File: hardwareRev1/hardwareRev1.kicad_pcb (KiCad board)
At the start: 2 copper layers, 0 parts

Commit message: board is almost done. Commiting before I destroy all my work...
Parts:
- added A1: GPSAnt, hardwareRev1:GPSAnt, F.Cu at (143.0, 84.0)
- added C1: C, Capacitors_SMD:C_0603, B.Cu at (167.7, 46.0)
- added C10: C, Capacitors_SMD:C_0603, F.Cu at (190.8, 41.8)
- added C11: C, Capacitors_SMD:C_0603, F.Cu at (178.8, 55.6)
- added C12: C, Capacitors_SMD:C_0603, B.Cu at (165.2, 56.8)
- added C13: C, Capacitors_SMD:C_0603, F.Cu at (175.1, 66.8)
- added C2: C, Capacitors_SMD:C_0603, F.Cu at (161.8, 62.6)
- added C3: C, Capacitors_SMD:C_0603, F.Cu at (175.1, 75.4)
- added C4: C, Capacitors_SMD:C_0603, F.Cu at (171.7, 72.6)
- added C5: C, Capacitors_SMD:C_0603, F.Cu at (180.0, 65.8)
- added C6: C, Capacitors_SMD:C_0603, F.Cu at (221.0, 53.0)
- added C7: CAPAPOL, Capacitors_SMD:C_0603, F.Cu at (221.0, 49.0)
- added C8: C, Capacitors_SMD:C_0603, B.Cu at (168.0, 76.0)
- added C9: C, Capacitors_SMD:C_0603, B.Cu at (171.0, 76.0)
- added D1: LED, LEDs:LED-0805, F.Cu at (167.6, 45.7)
- added D2: LED, LEDs:LED-0805, F.Cu at (169.3, 45.7)
- added D3: LED, LEDs:LED-0805, F.Cu at (171.1, 45.7)
- added D4: LED, LEDs:LED-0805, F.Cu at (172.8, 45.8)
- added D5: DIODE, Diodes_ThroughHole:Diode_DO-41_SOD81_Vertical_AnodeUp, F.Cu at (175.0, 46.0)
- added J1: MicroSD, Footprints:MICRO_SD_HINGE_AMP, B.Cu at (183.0, 72.0)
- added J2: SMA, hardwareRev1:SMA, F.Cu at (213.0, 74.0)
- added JMP1: SJMPOpen, SparkFun:SparkFun-SJ_2S-NO, B.Cu at (167.8, 48.6)
- added JMP2: SJMPOpen, SparkFun:SparkFun-SJ_2S-NO, F.Cu at (165.0, 45.0)
- added JMP3: SJMPOpen, SparkFun:SparkFun-SJ_2S-NO, F.Cu at (165.0, 47.0)
- added K1: PWMOut, Footprints:CONN_1x3, F.Cu at (146.8, 45.6)
- added K2: ADC1, Footprints:CONN_1x3, F.Cu at (146.8, 42.0)
- added P1: UART, Footprints:CONN_1x4, F.Cu at (148.0, 49.0)
- added P10: ID, Measurement_Points:Measurement_Point_Round-SMD-Pad_Small, B.Cu at (157.7, 47.2)
- added P2: I2C, Footprints:CONN_1x4, F.Cu at (148.0, 52.0)
- added P3: ADC2, Footprints:CONN_1x5, F.Cu at (143.8, 60.4)
- added P4: CONN_7, Footprints:CONN_1x7, F.Cu at (147.1, 63.0)
- added P5: CONN_5X2, hardwareRev1:CortexDebug, F.Cu at (192.2, 70.8)
- added P6: CONN_11X2, hardwareRev1:1.27mmPitchHeader11X2, F.Cu at (172.0, 42.0)
- added P7: GPSDM, Measurement_Points:Measurement_Point_Round-SMD-Pad_Small, F.Cu at (164.0, 67.0)
- added P8: GPSDP, Measurement_Points:Measurement_Point_Round-SMD-Pad_Small, F.Cu at (162.0, 67.0)
- added P9: USBPW, Measurement_Points:Measurement_Point_Round-SMD-Pad_Small, F.Cu at (161.7, 47.4)
- added Q1: MOS_P_NUM, SMD_Packages:SOT-323, B.Cu at (170.0, 72.0)
- added R1: R, Resistors_SMD:R_0603, F.Cu at (163.4, 62.6)
- added R10: R, Resistors_SMD:R_0603, F.Cu at (194.2, 41.5)
- added R11: R, Resistors_SMD:R_0603, F.Cu at (190.8, 39.8)
- added R12: R, Resistors_SMD:R_0603, F.Cu at (193.7, 74.8)
- added R13: R, Resistors_SMD:R_0603, B.Cu at (167.7, 73.0)
- added R2: R, Resistors_SMD:R_0603, F.Cu at (178.0, 49.0)
- added R3: R, Resistors_SMD:R_0603, F.Cu at (167.6, 49.2)
- added R4: R, Resistors_SMD:R_0603, F.Cu at (169.5, 49.2)
- added R5: R, Resistors_SMD:R_0603, F.Cu at (171.1, 49.2)
- added R6: R, Resistors_SMD:R_0603, F.Cu at (173.1, 49.2)
- added R7: R, Resistors_SMD:R_0603, F.Cu at (178.7, 70.8)
- added R8: R, Resistors_SMD:R_0603, F.Cu at (180.0, 68.0)
- added R9: R, Resistors_SMD:R_0603, F.Cu at (183.5, 65.8)
- added RF1: NEO7, hardwareRev1:NEO-7, F.Cu at (153.0, 83.0)
- added RF2: DRA818, dra818:DRA818, F.Cu at (182.0, 63.0)
- added S1: TAC_SWITCHSMD, SparkFun:SparkFun-TACTILE_SWITCH_SMD, B.Cu at (187.0, 61.0)
- added S2: TAC_SWITCHSMD, SparkFun:SparkFun-TACTILE_SWITCH_SMD, F.Cu at (156.4, 58.0)
- added U1: MKL26Z128VLH4, w_smd_lqfp:lqfp64, F.Cu at (171.0, 59.0)
- added U2: 24C16, Housings_SOIC:SOIC-8_3.9x4.9mm_Pitch1.27mm, B.Cu at (155.1, 59.0)
- added U3: MICRO-B_USB, USB:USB micro B female, F.Cu at (159.0, 42.0)
- added X1: CRYSTAL_ABM3C, open-project:CRYSTAL_ABM3C, F.Cu at (175.2, 70.8)
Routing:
- net GND: track 0.00 -> 333.9 mm, vias 0 -> 68
- net +3.3V: track 0.00 -> 171.9 mm, vias 0 -> 3
- net /internalSPI0MOSI: track 0.00 -> 47.7 mm, vias 0 -> 3
- net /DRAPttIRQ: track 0.00 -> 43.8 mm, vias 0 -> 2
- net /internalI2C0SCL: track 0.00 -> 42.5 mm, vias 0 -> 3
- net /DRAHLCSel: track 0.00 -> 42.2 mm, vias 0 -> 2
- net /DRATx: track 0.00 -> 39.5 mm, vias 0 -> 4
- net /DRAPD: track 0.00 -> 38.5 mm, vias 0 -> 2
- net /externalSPI1SCK: track 0.00 -> 36.9 mm, vias 0 -> 1
- net /GPSTX: track 0.00 -> 34.6 mm, vias 0 -> 2
- net /DRARx: track 0.00 -> 34.6 mm, vias 0 -> 2
- net /externalSPI1CS1: track 0.00 -> 34.5 mm, vias 0 -> 2
- net /externalPWMOut: track 0.00 -> 34.4 mm, vias 0 -> 2
- net /GPSRX: track 0.00 -> 34.2 mm, vias 0 -> 2
- net /externalSPI1PCS0: track 0.00 -> 32.4 mm, vias 0 -> 2
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- added copper zone on B.Cu, net GND
- added copper zone on F.Cu, net GND
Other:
- net class Default: clearance 0.2 -> 0.1524; trace_width 0.25 -> 0.1524
- rule pad_to_mask_clearance: 0 -> 0.2
- rule trace_clearance: 0.2 -> 0.1524
- rule trace_min: 0.2 -> 0.1524

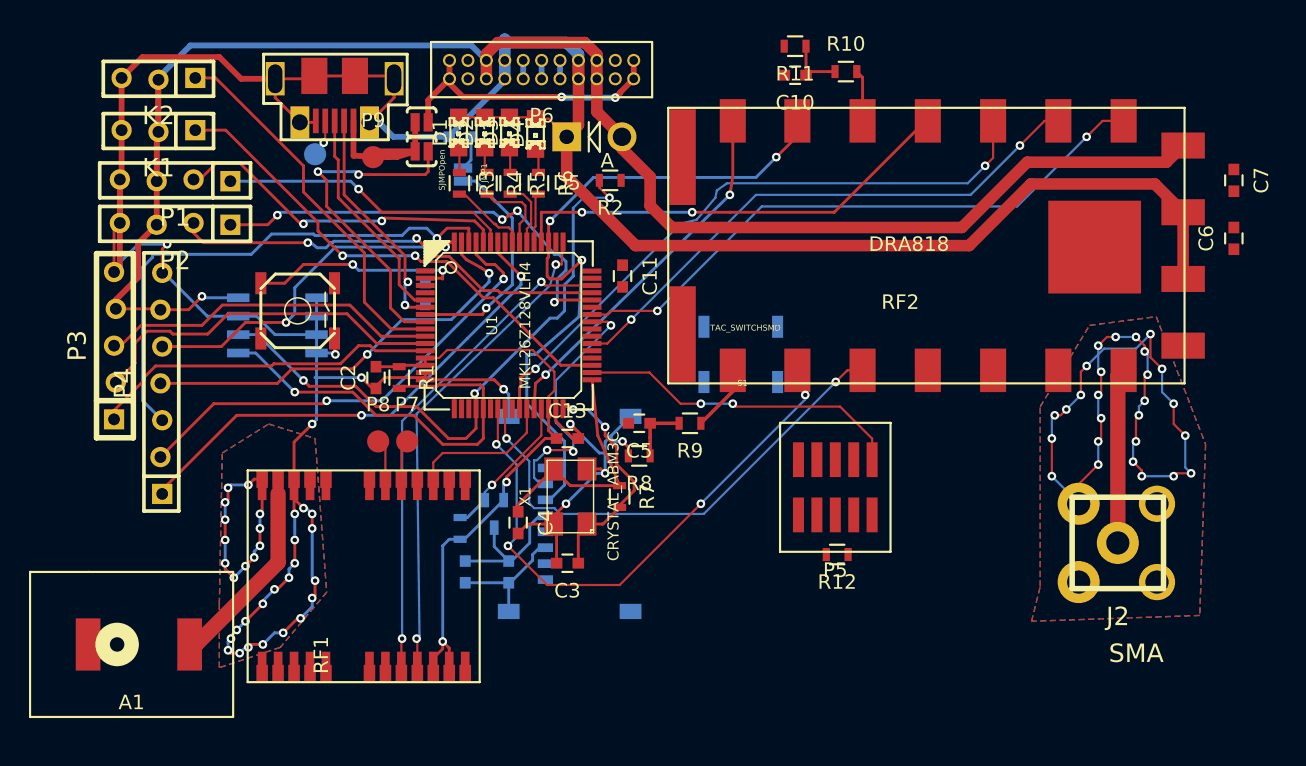
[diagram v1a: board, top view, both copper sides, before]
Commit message: went further.
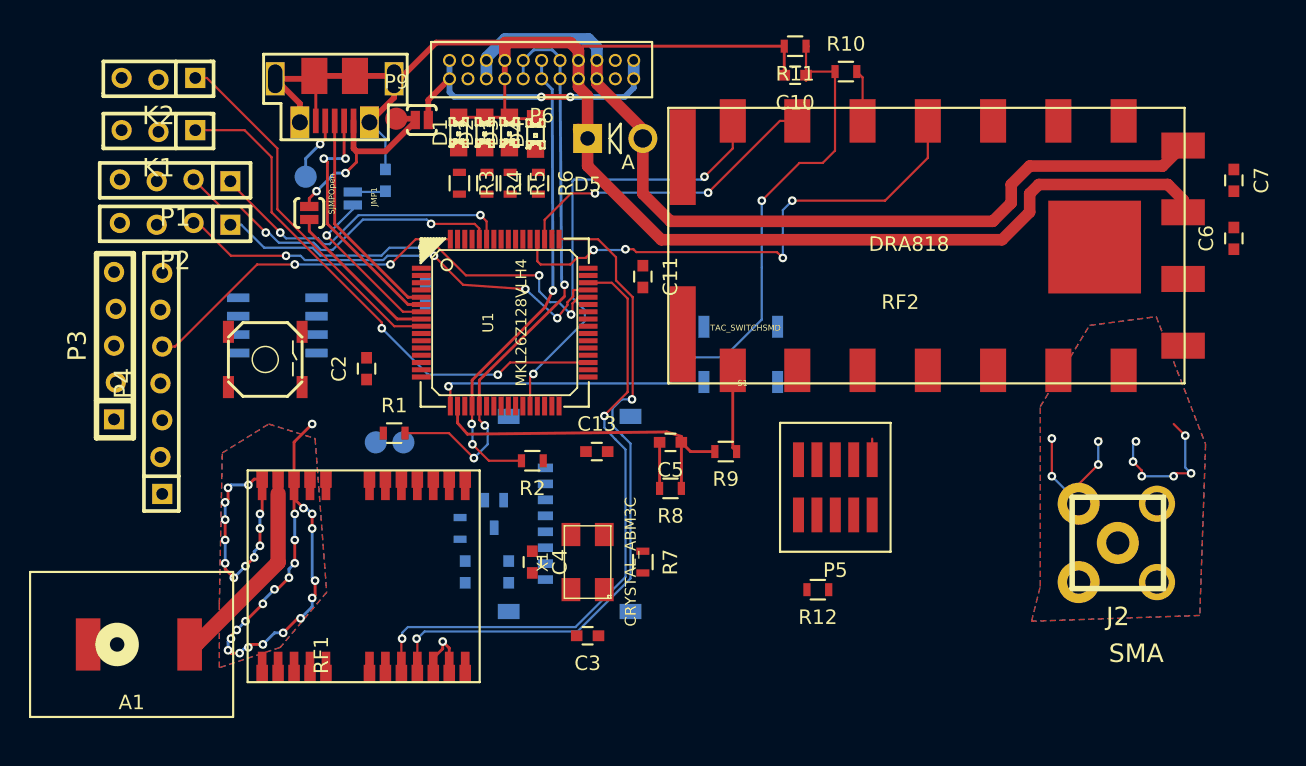
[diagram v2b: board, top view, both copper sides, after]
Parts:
- P7, P8: moved to B.Cu
- moved R2 20.1 mm to (172.6, 68.3)
- moved JMP3 8.84 mm to (157.2, 51.2), turned to 270 degrees
- moved JMP1 7.78 mm to (160.2, 50.2)
- moved C1 5.96 mm to (162.5, 49.0), turned to 270 degrees
- moved C3 5.19 mm to (176.4, 80.4)
- moved R7 4.79 mm to (180.2, 75.3)
- moved X1 4.67 mm to (176.4, 75.3)
- moved S2 4.03 mm to (154.2, 61.4)
- moved R1 3.85 mm to (163.1, 66.4), turned to 0 degrees
- moved R9 3.14 mm to (186.0, 67.7)
- moved R8 3.11 mm to (182.2, 70.2)
- moved P9 3.10 mm to (163.2, 44.8)
- moved C4 2.89 mm to (172.6, 75.3)
- moved R12 2.77 mm to (192.3, 77.2)
- moved C5 2.52 mm to (182.2, 67.1)
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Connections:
- P6 pad 10: /PWRSDA -> /internalI2C0SDA
- P6 pad 11: /PwrCLK -> /internalI2C0SCL
- P6 pad 12: /PwrCLK -> /internalI2C0SCL
- P6 pad 13: /PWRSDA -> /internalI2C0SDA
- P6 pad 14: /PWRSDA -> /internalI2C0SDA
- P6 pad 9: /PWRSDA -> /internalI2C0SDA
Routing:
- net GND: track 333.9 -> 183.8 mm, vias 68 -> 37
- net +3.3V: track 171.9 -> 65.0 mm, vias 3 -> 1
- net /DRAAFOut: track 4.75 -> 49.8 mm, vias 0 -> 2
- net /DRAPttIRQ: track 43.8 -> 0.00 mm, vias 2 -> 0
- net /DRAHLCSel: track 42.2 -> 0.00 mm, vias 2 -> 0
- net /DRATx: track 39.5 -> 0.00 mm, vias 4 -> 0
- net /DRAPD: track 38.5 -> 0.00 mm, vias 2 -> 0
- net /externalSPI1SCK: track 36.9 -> 0.00 mm, vias 1 -> 0
- net /DRARx: track 34.6 -> 0.00 mm, vias 2 -> 0
- net /externalSPI1CS1: track 34.5 -> 0.28 mm, vias 2 -> 0
- net /externalSPI1PCS0: track 32.4 -> 0.00 mm, vias 2 -> 0
- net /externalSPI1MOSI: track 29.3 -> 0.00 mm, vias 2 -> 0
- net /internalSPI0MOSI: track 47.7 -> 21.6 mm, vias 3 -> 2
- net /externalADC3: track 25.1 -> 0.00 mm
- net /externalADC4: track 24.2 -> 0.00 mm
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
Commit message: better routed it.
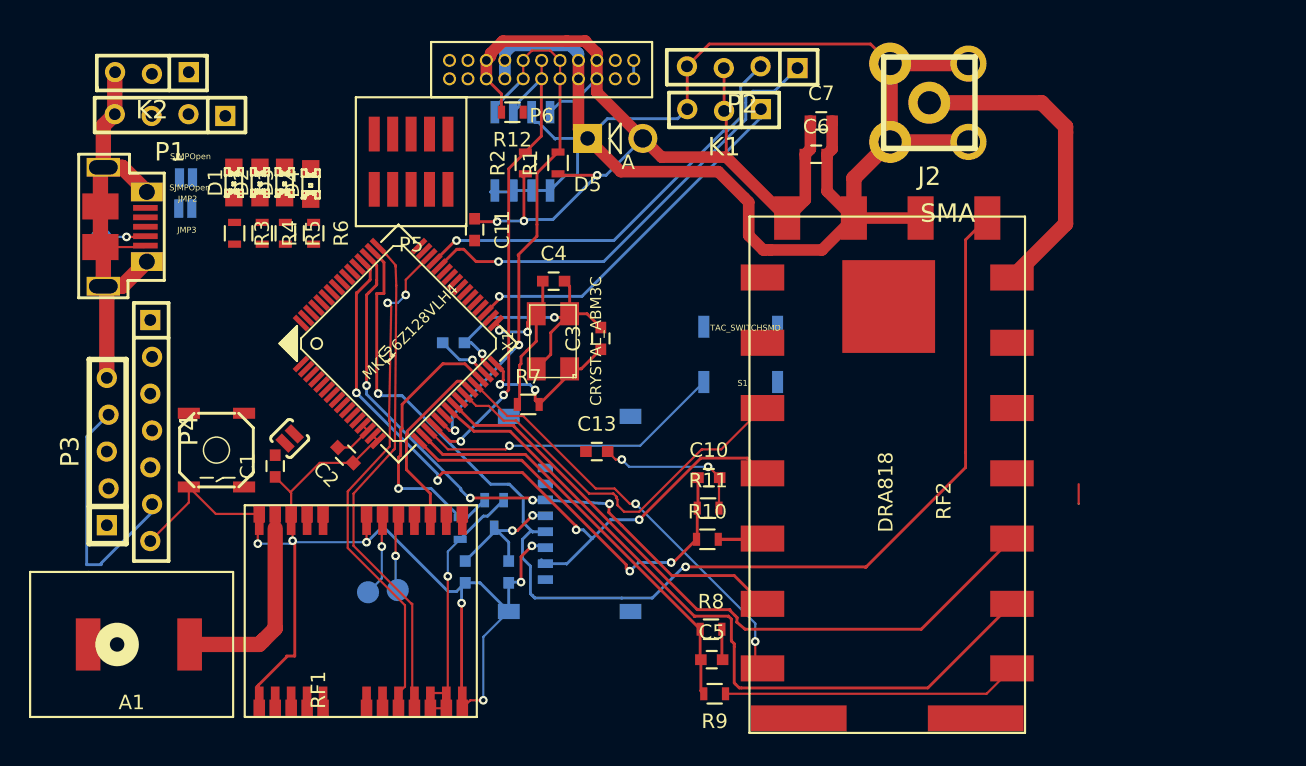
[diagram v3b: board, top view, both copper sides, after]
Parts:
- removed P9: USBPW, Measurement_Points:Measurement_Point_Round-SMD-Pad_Small
- C1, JMP1: moved to F.Cu
- JMP2, JMP3: moved to B.Cu
- moved P2 40.6 mm to (187.1, 41.2)
- moved R12 39.1 mm to (171.2, 44.3)
- moved K1 39.0 mm to (185.8, 44.1)
- moved P5 36.9 mm to (163.0, 48.4)
- moved RF2 34.4 mm to (206.6, 87.1), turned to 90 degrees
- moved R10 33.6 mm to (184.7, 73.8)
- moved J2 33.0 mm to (200.0, 43.6)
- moved R11 32.4 mm to (184.8, 71.6), turned to 0 degrees
- moved C6 29.4 mm to (192.2, 47.2), turned to 0 degrees
- moved C7 28.7 mm to (192.6, 44.9), turned to 0 degrees
- moved C10 28.4 mm to (184.8, 69.5), turned to 0 degrees
- moved R1 21.8 mm to (174.4, 47.8), turned to 90 degrees
- moved C1 21.1 mm to (154.9, 68.7), turned to 90 degrees
- moved U2 20.7 mm to (171.9, 47.0), turned to 90 degrees
- moved R2 20.5 mm to (172.2, 47.8), turned to 90 degrees
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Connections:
- RF1 pad 9: (no net) -> Net-(RF1-Pad9)
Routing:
- net /internalSPI0Clk: track 0.00 -> 83.9 mm, vias 0 -> 2
- net GND: track 183.8 -> 265.6 mm, vias 37 -> 11
- net /DRATx: track 0.00 -> 51.6 mm
- net +3.3V: track 65.0 -> 115.2 mm, vias 1 -> 5
- net /DRARx: track 0.00 -> 47.6 mm
- net /DRAPttIRQ: track 0.00 -> 27.2 mm
- net /externalADC1: track 25.1 -> 0.00 mm
- net /externalUART2TX: track 23.9 -> 0.00 mm, vias 2 -> 0
- net /externalSPI1MISO: track 22.9 -> 0.00 mm, vias 2 -> 0
- net /internalSPI0MOSI: track 21.6 -> 43.9 mm, vias 2 -> 4
- net Net-(J2-Pad1): track 0.00 -> 22.0 mm
- net /externalUART2RX: track 21.8 -> 0.00 mm, vias 2 -> 0
- net /DRAAFOut: track 49.8 -> 28.3 mm
- net /SW1: track 0.00 -> 21.4 mm, vias 0 -> 1
- net /SDPower: track 0.00 -> 20.2 mm, vias 0 -> 1
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- removed copper zone on B.Cu, net GND
- removed copper zone on F.Cu, net GND
